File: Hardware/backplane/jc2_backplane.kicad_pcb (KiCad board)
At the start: 2 copper layers, 97.5 x 102.5 mm, 15 parts, among them J0 JC2_DIN41612_02x32_AC, J1 JC2_DIN41612_02x32_AC, J2 JC2_DIN41612_02x32_AC, J3 JC2_DIN41612_02x32_AC, J4 Flat-cable, J5 POWER

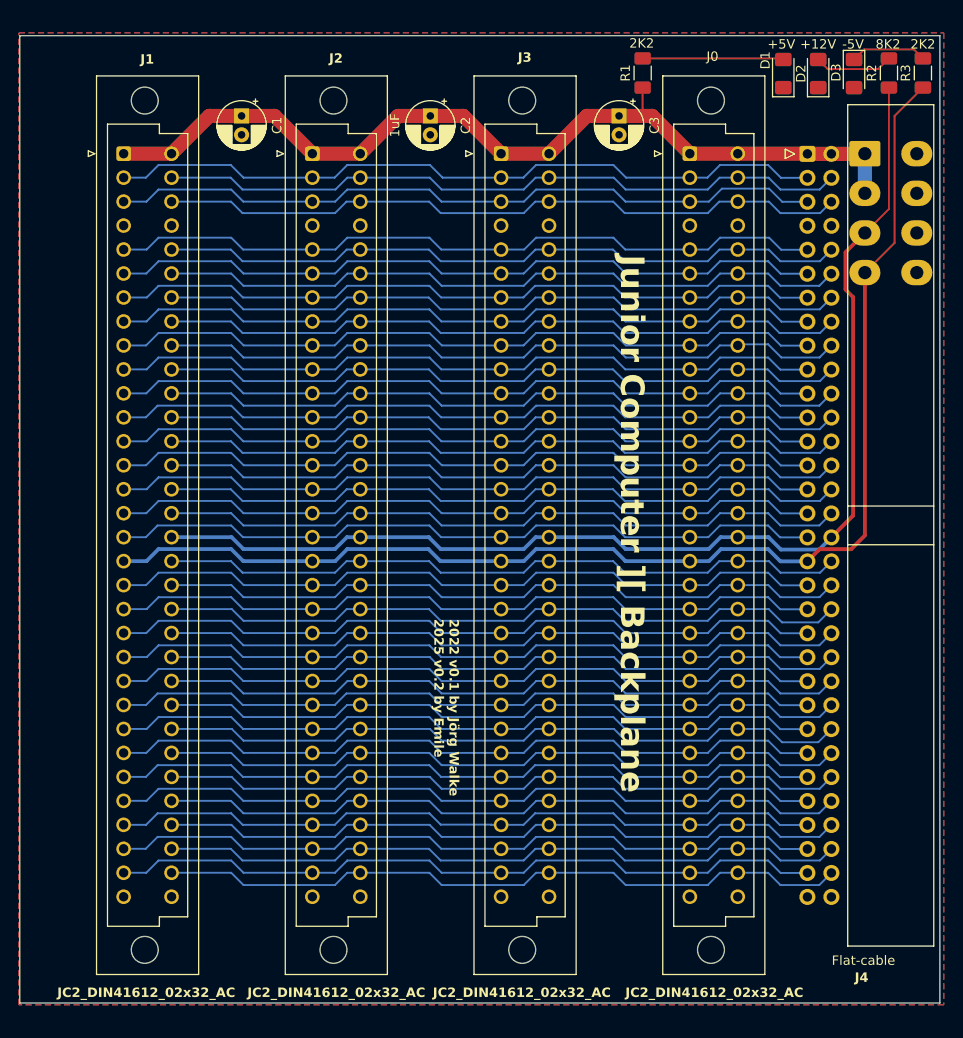
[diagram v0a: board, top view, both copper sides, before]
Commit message: Updates of mmu and backplane HW
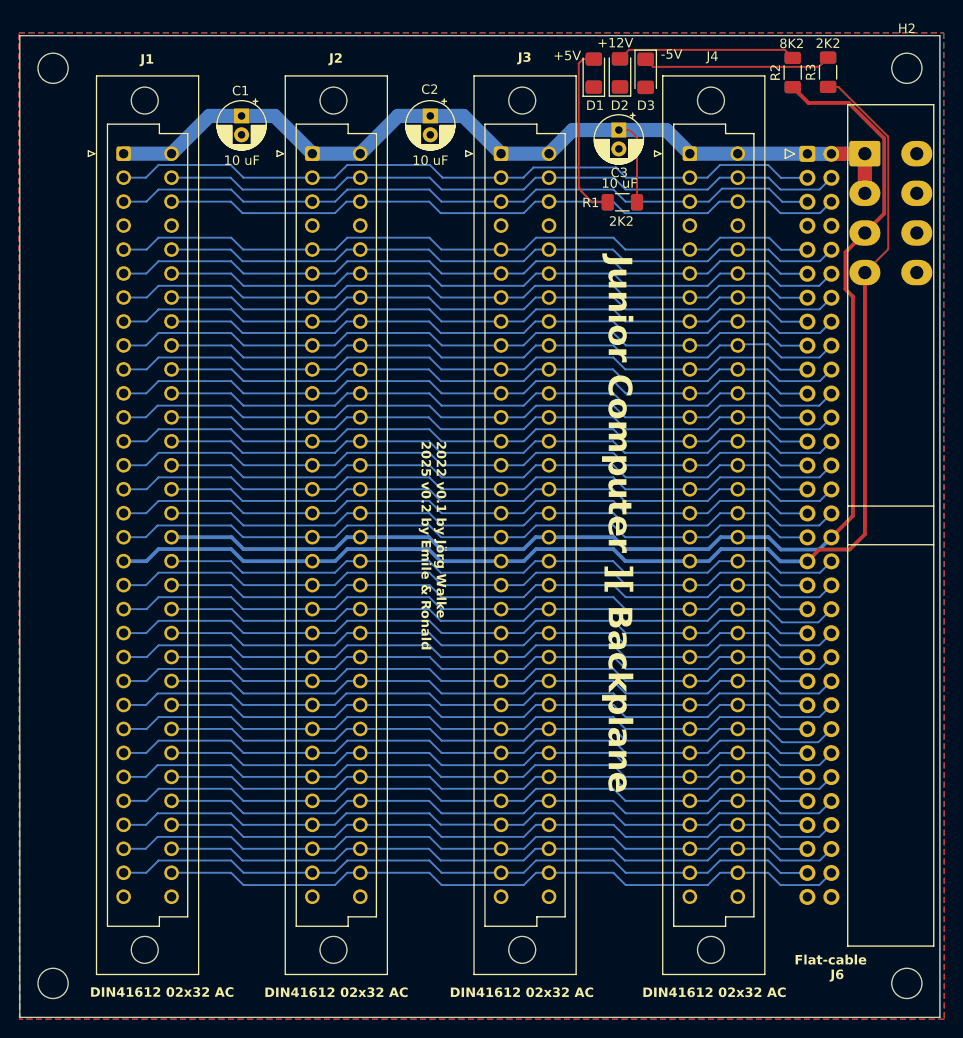
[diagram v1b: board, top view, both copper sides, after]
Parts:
- added H1: MountingHole, MountingHole:MountingHole_3.2mm_M3, F.Cu at (57.1, 40.2)
- added H2: MountingHole, MountingHole:MountingHole_3.2mm_M3, F.Cu at (147.6, 40.2)
- added H3: MountingHole, MountingHole:MountingHole_3.2mm_M3, F.Cu at (147.6, 137.2)
- added H4: MountingHole, MountingHole:MountingHole_3.2mm_M3, F.Cu at (57.1, 137.2)
- C1, C2, C3: value 1uF -> 10 uF
- J1, J2, J3: value JC2_DIN41612_02x32_AC -> DIN41612 02x32 AC
- J4: renamed from J0; value JC2_DIN41612_02x32_AC -> DIN41612 02x32 AC
- moved D3 22.1 mm to (119.9, 40.8)
- moved D2 21.0 mm to (117.2, 40.7)
- moved D1 20.1 mm to (114.4, 40.8)
- moved R1 13.9 mm to (117.5, 54.5), turned to 180 degrees
- moved R2 10.2 mm to (135.5, 40.7)
- moved R3 10.1 mm to (139.2, 40.7)
- moved C3 1.50 mm to (117.1, 46.8)
- renumbered J4 to J6
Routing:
- net Net-(D3-K): track 8.14 -> 20.1 mm
- net Net-(D2-A): track 8.39 -> 19.1 mm
- net +5V: track 95.7 -> 104.1 mm
- net +12V: track 125.0 -> 131.3 mm
- net Net-(D1-A): track 15.0 -> 18.7 mm
- net -5V: track 133.9 -> 135.7 mm
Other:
- board size 97.5 x 102.5 mm -> 97.5 x 104 mm
- board text added: "2022 v0.1 by Jörg Walke 2025 v0.2 by Emile & Ronald"
- board text added: "GND +5V GND +5V GND +12V GND -5V"
- board text removed: "2022 v0.1 by Jörg Walke 2025 v0.2 by Emile"
